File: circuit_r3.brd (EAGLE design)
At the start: 57.3 x 43.2 mm, 24 parts, among them IC1 7805DT, U1 MCP4725, U2 MB85RC256VPF-G-JNERE2, U4 ATMEGA328P_VQFNVQFN, Y1 16MHz

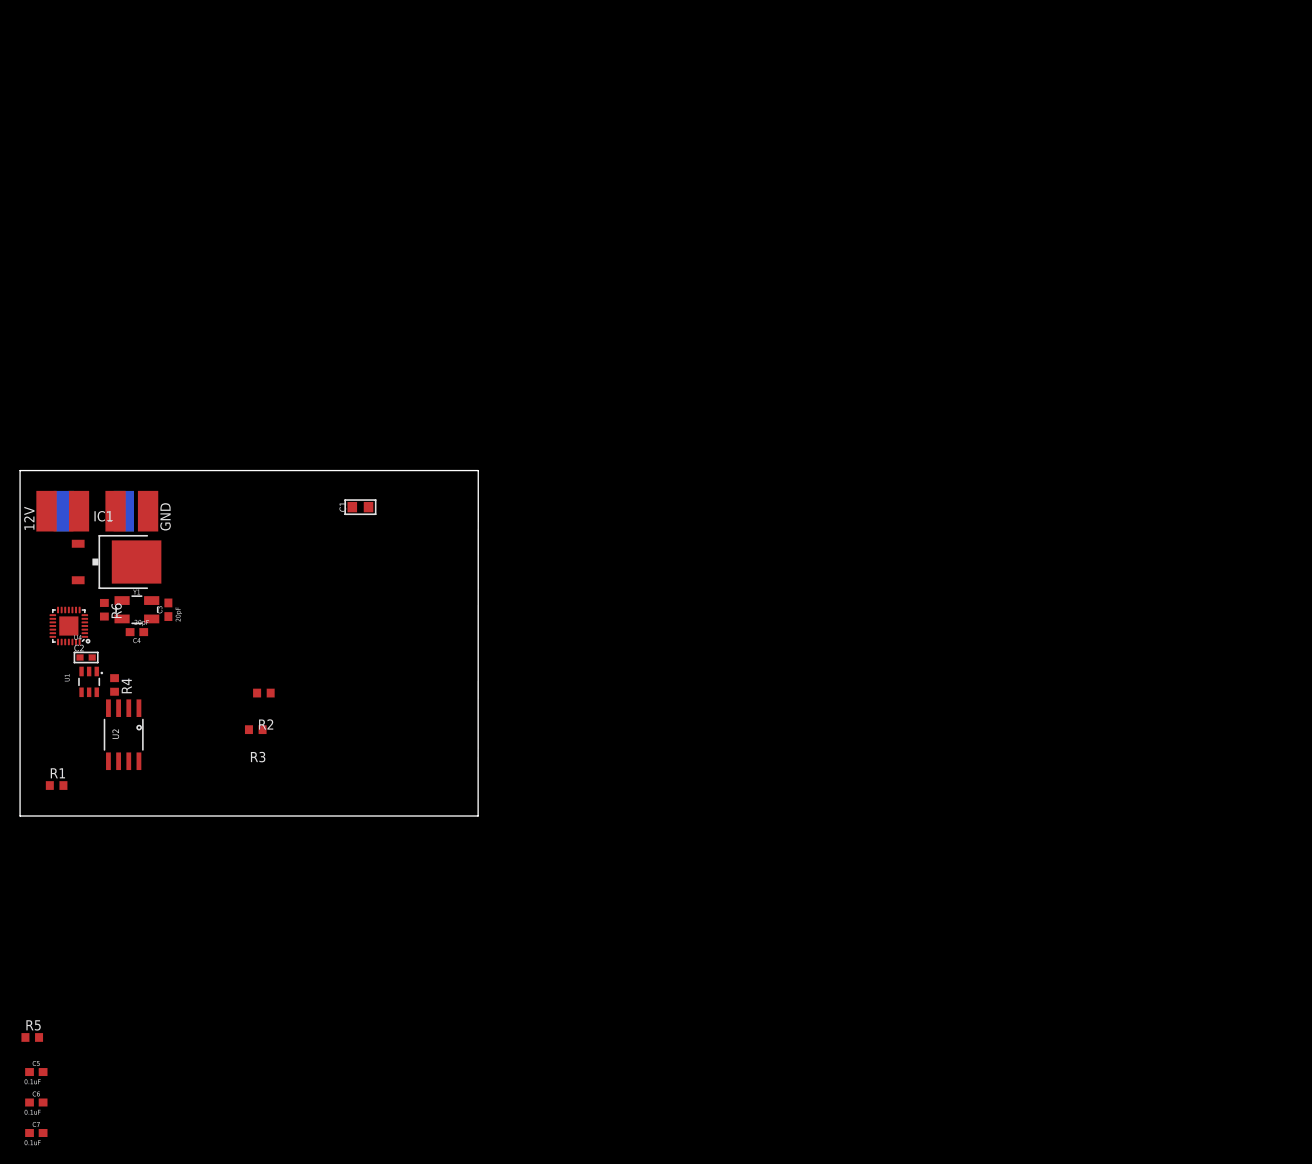
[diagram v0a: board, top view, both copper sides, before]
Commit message: Oooh, getting close.
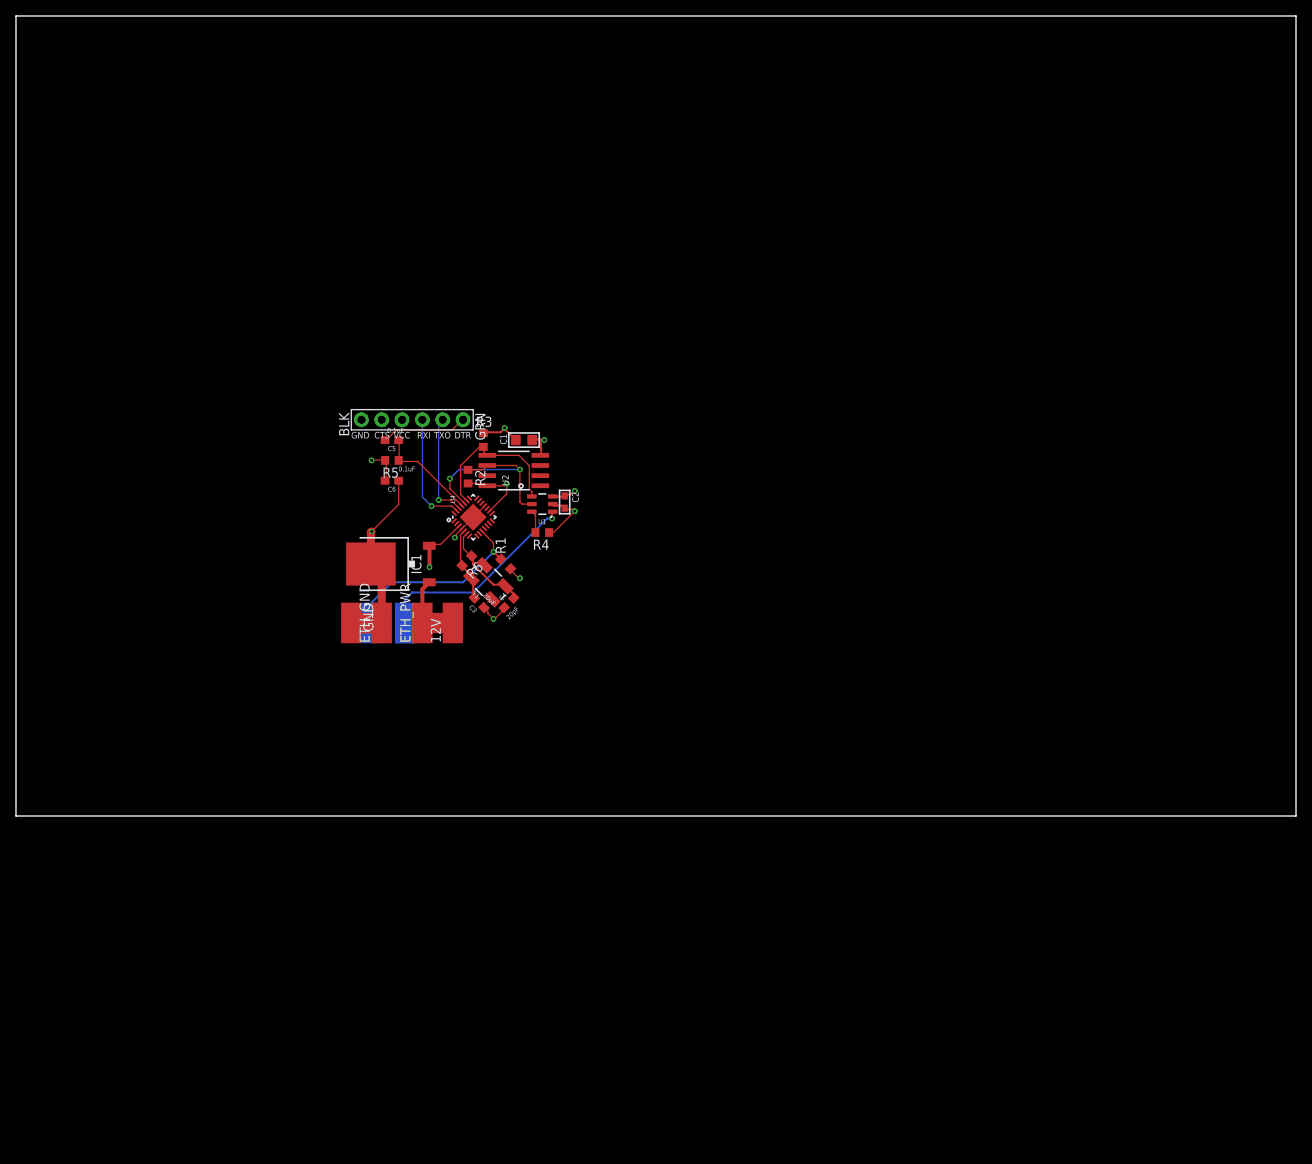
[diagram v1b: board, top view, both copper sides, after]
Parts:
- removed C7: 0.1uF, custom:0603
- added J1: (no value), SparkFun-Connectors:6_PIN_SERIAL_TARGET_SIDE_W_SILK
- moved C5 90.6 mm to (47.0, 47.0), turned to 180 degrees
- moved C6 89.5 mm to (47.0, 41.9), turned to 180 degrees
- moved R5 85.0 mm to (47.0, 44.5), turned to 180 degrees
- moved C2 62.9 mm to (68.6, 39.2), turned to 270 degrees
- moved R1 62.6 mm to (61.2, 31.5), turned to 315 degrees
- moved U1 60.8 mm to (65.8, 39.0), turned to 270 degrees
- moved U2 58.9 mm to (62.2, 43.2), turned to 90 degrees
- moved R4 56.8 mm to (65.8, 35.4), turned to 180 degrees
- moved 12V 52.7 mm to (54.6, 24.1)
- moved U4 50.4 mm to (57.1, 35.6), turned to 45 degrees
- moved C4 46.7 mm to (61.6, 26.6), turned to 45 degrees
- moved R3 46.0 mm to (58.4, 47.0), turned to 90 degrees
- moved R6 45.7 mm to (56.4, 31.9), turned to 225 degrees
- moved ETH_PWR 45.1 mm to (50.8, 24.1)
- moved Y1 44.1 mm to (59.1, 29.2), turned to 135 degrees
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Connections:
- removed net AREF: C7.1, U4.17
- new net RXI: J1.P$2, U4.26
- new net TXO: J1.P$3, U4.27
- net DTR: now also J1.P$1
- net GND: now also J1.P$5, J1.P$6; no longer C7.2
- net VCC: now also J1.P$4
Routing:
- net GND: track 0.00 -> 48.2 mm, vias 0 -> 5
- net VCC: track 0.00 -> 31.7 mm, vias 0 -> 6
- net OUT: track 0.00 -> 26.4 mm, vias 0 -> 1
- net SCL: track 0.00 -> 26.1 mm, vias 0 -> 2
- net ETH: track 0.00 -> 24.9 mm, vias 0 -> 1
- net SDA: track 0.00 -> 19.5 mm
- net TXO: track 0.00 -> 14.7 mm, vias 0 -> 1
- net RXI: track 0.00 -> 13.3 mm, vias 0 -> 1
- net RESET: track 0.00 -> 12.9 mm
- net XT2: track 0.00 -> 11.7 mm
- net DTR: track 0.00 -> 10.8 mm
- net XT1: track 0.00 -> 9.59 mm
- net VIN: track 0.00 -> 9.25 mm
- net PD_L: track 0.00 -> 2.79 mm
- added copper zone on layer 2, net GND
- added copper zone on layer 15, net VCC
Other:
- board size 57.3 x 43.2 mm -> 160 x 100 mm
